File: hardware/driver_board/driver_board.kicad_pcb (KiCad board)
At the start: 2 copper layers, 155 x 100 mm, 103 parts, among them J1 796949-2, J2 796949-2, J3 796949-2, J4 796949-2, J5 Adafruit_1979, Q1 Toshiba_TK4R3E06PL, Q2 Toshiba_TK4R3E06PL, Q3 Toshiba_TK4R3E06PL, Q4 Toshiba_TK4R3E06PL, Q5 Toshiba_TK4R3E06PL, Q6 Toshiba_TK4R3E06PL, Q7 Toshiba_TK4R3E06PL, Q8 Toshiba_TK4R3E06PL, U1 HCPL-2631, U2 HCPL-2631, U3 IR2110, U4 IR2110, U5 IR2110, U6 IR2110, U7 LM7812_TO220, U8 MP1584EN

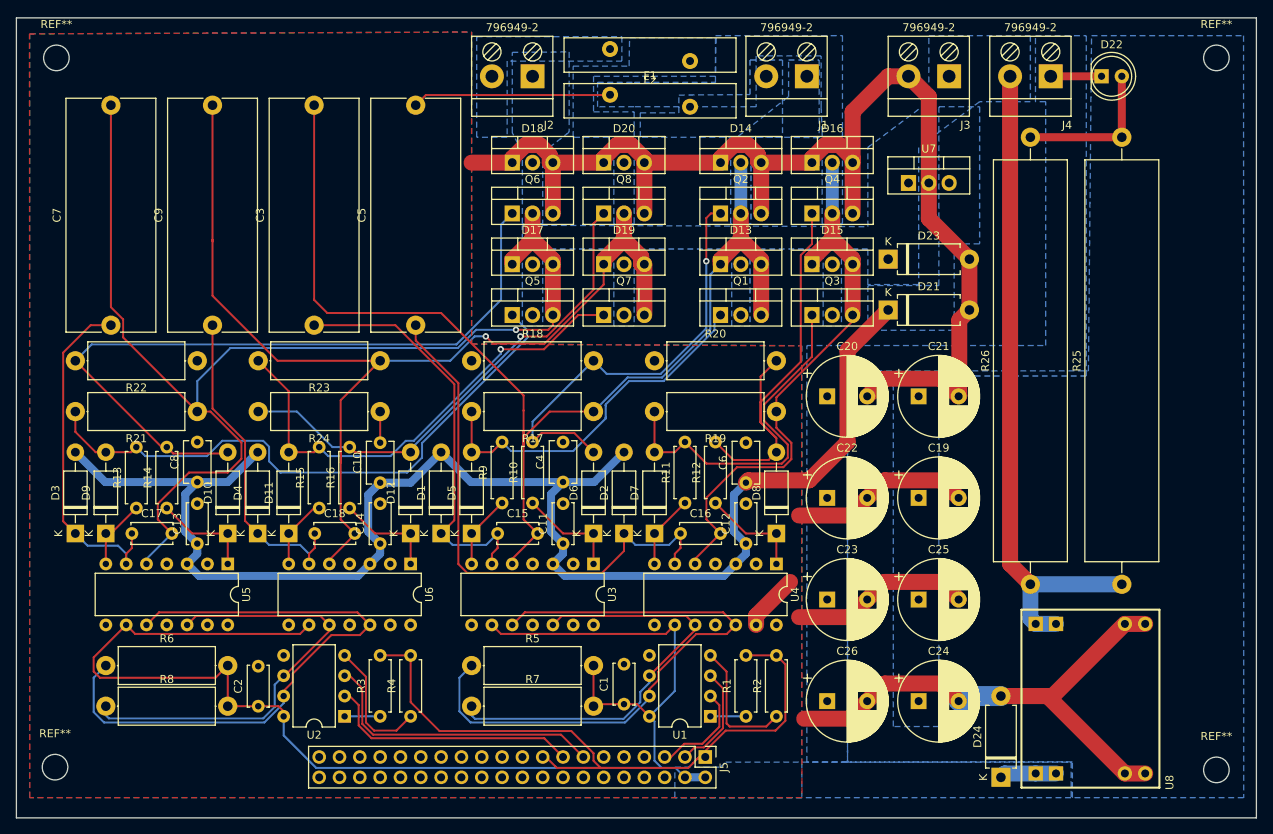
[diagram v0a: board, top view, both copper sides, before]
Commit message: final update
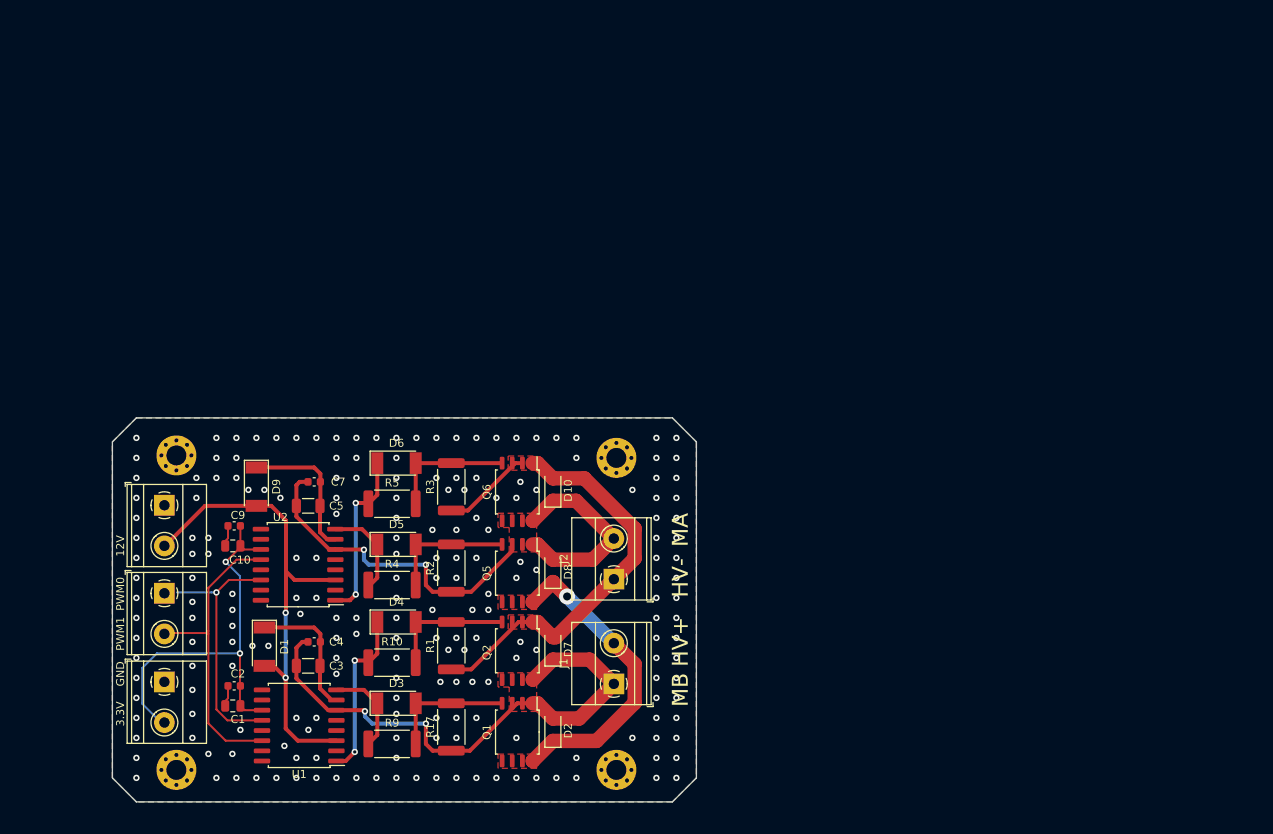
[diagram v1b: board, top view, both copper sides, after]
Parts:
- removed C11, C12, C13, C14, C15, C16, C17, C18: 100nF, driver_board:C_Disc_D5.0mm_W2.5mm_P5.00mm
- removed C19, C20, C21, C22, C23, C24, C25, C26: 1000uF, driver_board:CP_Radial_D10.0mm_P5.00mm
- removed C6, C8: 22uF, driver_board:C_Disc_D5.1mm_W3.2mm_P5.00mm
- removed D11, D12: UF4007, Diode_THT:D_DO-41_SOD81_P10.16mm_Horizontal
- removed D13, D14, D15, D16, D17, D18, D19, D20: NTST30120CTG, driver_board:NTST30120CTG
- removed D21, D23, D24: D_TVS, driver_board:D_DO-15_P10.16mm_Horizontal
- removed D22: LED, driver_board:LED_D5.0mm_PRECAHRGE
- removed F1, F2: Bel Fuse 0ZRS1000FF1A, driver_board:RV_Disc_D21.5mm_W4.3mm_P10mm
- removed Q3, Q4, Q7, Q8: Toshiba_TK4R3E06PL, driver_board:TK4R3E06RL
- removed R11, R12, R13, R14, R15, R16: 10R, driver_board:R_Axial_DIN0207_L6.3mm_D2.5mm_P7.62mm_Horizontal
- removed R18, R19, R20, R21, R22, R23, R24, R6, R7, R8: 1kR, driver_board:R_Axial_DIN0414_L11.9mm_D4.5mm_P15.24mm_Horizontal
- removed R25, R26: 1kR, driver_board:R_Axial_Power_L50.0mm_W9.0mm_P55.88mm
- removed the REF** at (196.6, 157.2)
- removed the REF** at (51.4, 156.8)
- removed the REF** at (196.6, 68.2)
- removed the REF** at (51.6, 68.2)
- removed U3, U4, U5, U6: IR2110, Package_DIP:DIP-14_W7.62mm
- removed U7: LM7812_TO220, Package_TO_SOT_THT:TO-220-3_Vertical
- removed U8: MP1584EN, driver_board:MP1584
- added REF**: MountingHole_2.5mm_Pad_Via, MountingHole:MountingHole_2.5mm_Pad_Via, F.Cu at (121.6, 118.2)
- added REF**: MountingHole_2.5mm_Pad_Via, MountingHole:MountingHole_2.5mm_Pad_Via, F.Cu at (121.6, 157.2)
- added REF**: MountingHole_2.5mm_Pad_Via, MountingHole:MountingHole_2.5mm_Pad_Via, F.Cu at (66.6, 157.2)
- added REF**: MountingHole_2.5mm_Pad_Via, MountingHole:MountingHole_2.5mm_Pad_Via, F.Cu at (66.6, 117.9)
- C1: value 100nF -> 22uF; footprint driver_board:C_Disc_D5.0mm_W2.5mm_P5.00mm -> Capacitor_SMD:C_0805_2012Metric
- C10: footprint driver_board:C_Disc_D5.1mm_W3.2mm_P5.00mm -> Capacitor_SMD:C_0805_2012Metric
- C2: footprint driver_board:C_Disc_D5.0mm_W2.5mm_P5.00mm -> Capacitor_SMD:C_0603_1608Metric
- C3, C5: value 22uF -> C; footprint driver_board:C_Rect_L29.0mm_W11.0mm_P27.50mm_MKT -> Capacitor_SMD:C_1206_3216Metric
- C4: value 22uF -> 100nF; footprint driver_board:C_Disc_D5.1mm_W3.2mm_P5.00mm -> Capacitor_SMD:C_0603_1608Metric
- C7, C9: value 22uF -> 100nF; footprint driver_board:C_Rect_L29.0mm_W11.0mm_P27.50mm_MKT -> Capacitor_SMD:C_0603_1608Metric
- D1, D3, D4, D5, D6, D9: value UF4007 -> SUF4007; footprint Diode_THT:D_DO-41_SOD81_P10.16mm_Horizontal -> Diode_SMD:D_MELF
- D10, D2, D7, D8: value UF4007 -> 1N4007; footprint Diode_THT:D_DO-41_SOD81_P10.16mm_Horizontal -> Diode_SMD:D_SOD-123F
- J1, J2, J3, J4: footprint driver_board:796949-2 -> TerminalBlock_Phoenix:TerminalBlock_Phoenix_MKDS-1,5-2-5.08_1x02_P5.08mm_Horizontal
- J5: value Adafruit_1979 -> 796949-2; footprint driver_board:Adafruit_1979 -> TerminalBlock_Phoenix:TerminalBlock_Phoenix_MKDS-1,5-2-5.08_1x02_P5.08mm_Horizontal
- Q1, Q2, Q5, Q6: value Toshiba_TK4R3E06PL -> TPH4R008NH,L1Q(M; footprint driver_board:TK4R3E06RL -> driver_board:TPH4R008NH,L1Q(M
- R1, R2, R3: value 300R -> 1kR; footprint driver_board:R_Axial_DIN0207_L6.3mm_D2.5mm_P7.62mm_Horizontal -> Resistor_SMD:R_2512_6332Metric
- R10, R9: footprint driver_board:R_Axial_DIN0207_L6.3mm_D2.5mm_P7.62mm_Horizontal -> Resistor_SMD:R_2512_6332Metric
- R17: footprint driver_board:R_Axial_DIN0414_L11.9mm_D4.5mm_P15.24mm_Horizontal -> Resistor_SMD:R_2512_6332Metric
- R4: value 300R -> 10R; footprint driver_board:R_Axial_DIN0207_L6.3mm_D2.5mm_P7.62mm_Horizontal -> Resistor_SMD:R_2512_6332Metric
- R5: value 1kR -> 10R; footprint driver_board:R_Axial_DIN0414_L11.9mm_D4.5mm_P15.24mm_Horizontal -> Resistor_SMD:R_2512_6332Metric
- U1, U2: value HCPL-2631 -> IR2110S; footprint Package_DIP:DIP-8_W7.62mm -> Package_SO:SOIC-16W_7.5x10.3mm_P1.27mm
- moved J4 128.3 mm to (65.1, 135.1), turned to 270 degrees
- moved J3 111.8 mm to (65.1, 124.1), turned to 270 degrees
- moved J1 79.7 mm to (121.3, 146.4), turned to 90 degrees
- moved J5 68.3 mm to (65.1, 146.2)
- moved J2 63.7 mm to (121.3, 133.3), turned to 90 degrees
- moved Q2 60.3 mm to (109.2, 142.3), turned to 270 degrees
- moved Q1 58.0 mm to (109.2, 152.5), turned to 270 degrees
- moved U1 51.4 mm to (82.0, 151.6)
- moved C1 48.9 mm to (73.7, 149.2), turned to 180 degrees
- moved D3 45.4 mm to (94.1, 148.9), turned to 0 degrees
- moved R2 44.7 mm to (101.0, 132.0)
- moved R17 43.3 mm to (101.0, 151.8), turned to 90 degrees
- moved C3 42.6 mm to (83.1, 144.2), turned to 180 degrees
- moved D10 41.0 mm to (113.7, 122.1)
- moved R1 37.9 mm to (101.0, 141.7)
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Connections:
- C1 pad 1: +5V -> +3V3
- C10 pad 1: +12V -> +3V3
- C2 pad 1: +5V -> +3V3
- C3 pad 1: Net-(C15-Pad1) -> Net-(C3-Pad1)
- C3 pad 2: Net-(C15-Pad2) -> M+
- C4 pad 1: +12V -> Net-(C3-Pad1)
- C4 pad 2: GND -> M+
- C5 pad 1: Net-(C16-Pad1) -> Net-(C5-Pad1)
- C5 pad 2: Net-(C16-Pad2) -> M-
- C7 pad 1: Net-(C17-Pad1) -> Net-(C5-Pad1)
- C7 pad 2: Net-(C17-Pad2) -> M-
- C9 pad 1: Net-(C18-Pad1) -> +3V3
- C9 pad 2: Net-(C18-Pad2) -> GND
- D1 pad 1: Net-(C15-Pad1) -> Net-(C3-Pad1)
- D10 pad 1: Net-(D10-Pad1) -> M-
- D10 pad 2: Net-(D10-Pad2) -> HV-
- D2 pad 1: Net-(C16-Pad1) -> HV+
- D2 pad 2: +12V -> M+
- D3 pad 1: Net-(C17-Pad1) -> Net-(D3-Pad1)
- D3 pad 2: +12V -> Net-(D3-Pad2)
- D4 pad 1: Net-(C18-Pad1) -> Net-(D4-Pad1)
- D4 pad 2: +12V -> Net-(D4-Pad2)
- D7 pad 1: Net-(D7-Pad1) -> M+
- D7 pad 2: Net-(D7-Pad2) -> HV-
- D8 pad 1: Net-(D8-Pad1) -> HV+
- D8 pad 2: Net-(D8-Pad2) -> M-
- D9 pad 1: Net-(D9-Pad1) -> Net-(C5-Pad1)
- D9 pad 2: Net-(D9-Pad2) -> +12V
- J1 pad 1: Net-(C15-Pad2) -> M+
- J1 pad 2: Net-(F1-Pad1) -> HV+
- J2 pad 1: Net-(C17-Pad2) -> HV-
- J2 pad 2: Net-(F2-Pad1) -> M-
- J3 pad 1: +24V -> Net-(J3-Pad1)
- J3 pad 2: GND -> +12V
- J4 pad 1: Net-(C19-Pad1) -> PWM0
- J4 pad 2: +24V -> PWM1
- J5 pad 1: +3V3 -> GND
- J5 pad 2: +5V -> +3V3
- Q1 pad 1: Net-(D5-Pad2) -> M+
- Q1 pad 2: +24V -> Net-(D3-Pad2)
- Q1 pad 3: Net-(C15-Pad2) -> HV+
- Q2 pad 1: Net-(D6-Pad2) -> HV-
- Q2 pad 2: Net-(C15-Pad2) -> Net-(D4-Pad2)
- Q2 pad 3: GND -> M+
- Q5 pad 1: Net-(D9-Pad2) -> M-
- Q5 pad 2: +24V -> Net-(D5-Pad2)
- Q5 pad 3: Net-(C17-Pad2) -> HV+
- Q6 pad 1: Net-(D10-Pad2) -> HV-
- Q6 pad 2: Net-(C17-Pad2) -> Net-(D6-Pad2)
- Q6 pad 3: GND -> M-
- R1 pad 1: Net-(R1-Pad1) -> HV-
- R1 pad 2: +3V3 -> Net-(D4-Pad2)
- R10 pad 1: Net-(D6-Pad1) -> Net-(D4-Pad1)
- R10 pad 2: Net-(D6-Pad2) -> Net-(D4-Pad2)
- R17 pad 1: Net-(C15-Pad2) -> M+
- R17 pad 2: Net-(D5-Pad2) -> Net-(D3-Pad2)
- R2 pad 1: Net-(R2-Pad1) -> M-
- R2 pad 2: +3V3 -> Net-(D5-Pad2)
- R3 pad 1: Net-(R3-Pad1) -> HV-
- R3 pad 2: +3V3 -> Net-(D6-Pad2)
- R4 pad 1: Net-(R4-Pad1) -> Net-(D5-Pad1)
- R4 pad 2: +3V3 -> Net-(D5-Pad2)
- R5 pad 1: Net-(R5-Pad1) -> Net-(D6-Pad1)
- R5 pad 2: +5V -> Net-(D6-Pad2)
- R9 pad 1: Net-(D5-Pad1) -> Net-(D3-Pad1)
- R9 pad 2: Net-(D5-Pad2) -> Net-(D3-Pad2)
- U1 pad 1: Net-(R1-Pad1) -> Net-(D4-Pad1)
- U1 pad 2: GPIO3 -> GND
- U1 pad 3: GPIO2 -> +12V
- U1 pad 4: Net-(R2-Pad1) -> Net-(U1-Pad4)
- U1 pad 5: GND -> Net-(U1-Pad5)
- U1 pad 6: Net-(R7-Pad1) -> M+
- U1 pad 7: Net-(R5-Pad1) -> Net-(C3-Pad1)
- U1 pad 8: +5V -> Net-(D3-Pad1)
- U2 pad 1: Net-(R3-Pad1) -> Net-(D6-Pad1)
- U2 pad 2: GPIO22 -> GND
- U2 pad 3: GPIO27 -> +12V
- U2 pad 4: Net-(R4-Pad1) -> Net-(U2-Pad4)
- U2 pad 5: GND -> Net-(U2-Pad5)
- U2 pad 6: Net-(R8-Pad1) -> M-
- U2 pad 7: Net-(R6-Pad1) -> Net-(C5-Pad1)
- U2 pad 8: +5V -> Net-(D5-Pad1)
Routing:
- net GND: track 282.8 -> 5.29 mm, vias 0 -> 209
- net +5V: track 183.0 -> 0.00 mm
- net Net-(C17-Pad2): track 145.2 -> 0.00 mm, vias 1 -> 0
- net Net-(C15-Pad2): track 145.1 -> 0.00 mm
- net Net-(C18-Pad2): track 132.5 -> 0.00 mm, vias 1 -> 0
- net +12V: track 191.2 -> 60.9 mm, vias 0 -> 2
- net Net-(C16-Pad2): track 96.1 -> 0.00 mm
- net Net-(D10-Pad2): track 91.7 -> 0.00 mm
- net +24V: track 83.7 -> 0.00 mm
- net Net-(R6-Pad1): track 77.3 -> 0.00 mm
- net Net-(R5-Pad1): track 77.0 -> 0.00 mm
- net Net-(D9-Pad2): track 76.2 -> 0.00 mm
- net Net-(C16-Pad1): track 68.9 -> 0.00 mm
- net M+: track 0.00 -> 68.4 mm, vias 0 -> 2
- net M-: track 0.00 -> 66.0 mm, vias 0 -> 2
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- added copper zone on F.Cu, net HV+
- added copper zone on F.Cu, net HV-
- added copper zone on F.Cu, net M+
- added copper zone on F.Cu, net M-
- removed copper zone on B.Cu, net +12V
- removed copper zone on B.Cu, net +24V
- removed copper zone on B.Cu, net +5V
- removed copper zone on B.Cu, net Net-(C15-Pad2)
- removed copper zone on B.Cu, net Net-(C16-Pad2)
- removed copper zone on B.Cu, net Net-(C17-Pad2)
- removed copper zone on B.Cu, net Net-(C18-Pad2)
- removed copper zone on B.Cu, net Net-(C19-Pad1)
- removed copper zone on B.Cu, net Net-(F1-Pad1)
- removed copper zone on B.Cu, net Net-(F2-Pad1)
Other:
- board size 155 x 100 mm -> 73 x 48 mm
- board text added: "12V"
- board text added: "3.3V"
- board text added: "GND"
- board text added: "HV+"
- board text added: "HV-"
- board text added: "MA"
- board text added: "MB"
- board text added: "PWM0"
- board text added: "PWM1"
